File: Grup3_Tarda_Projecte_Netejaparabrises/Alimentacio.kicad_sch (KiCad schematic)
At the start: 12 parts, among them J1 Screw_Terminal_01x02, U1 LM1117-ADJ, U1 LM1117MP-5.0

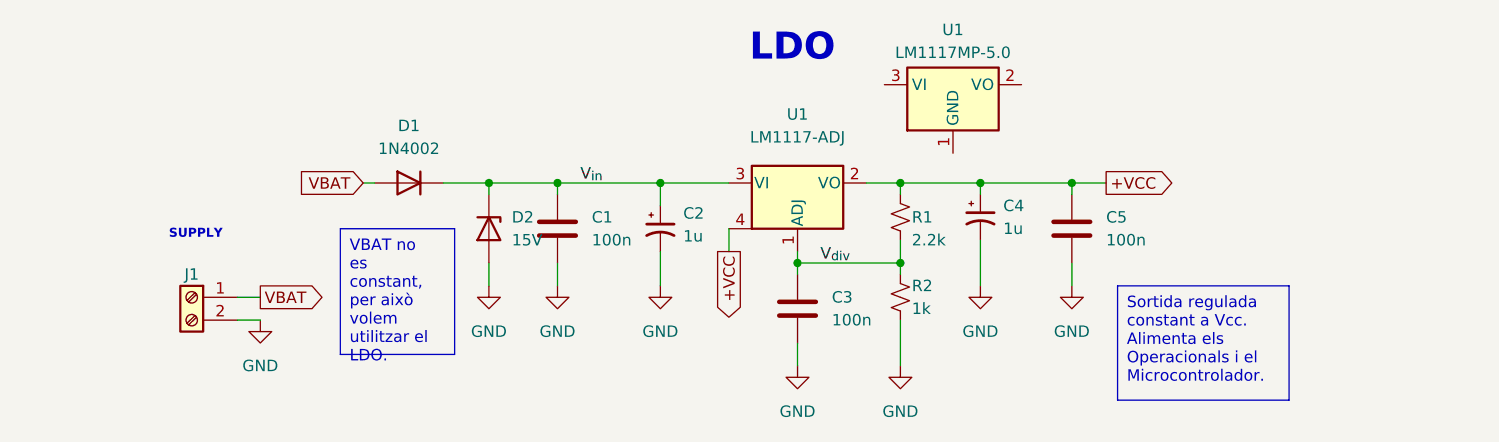
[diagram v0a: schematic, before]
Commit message: canvis esquematic
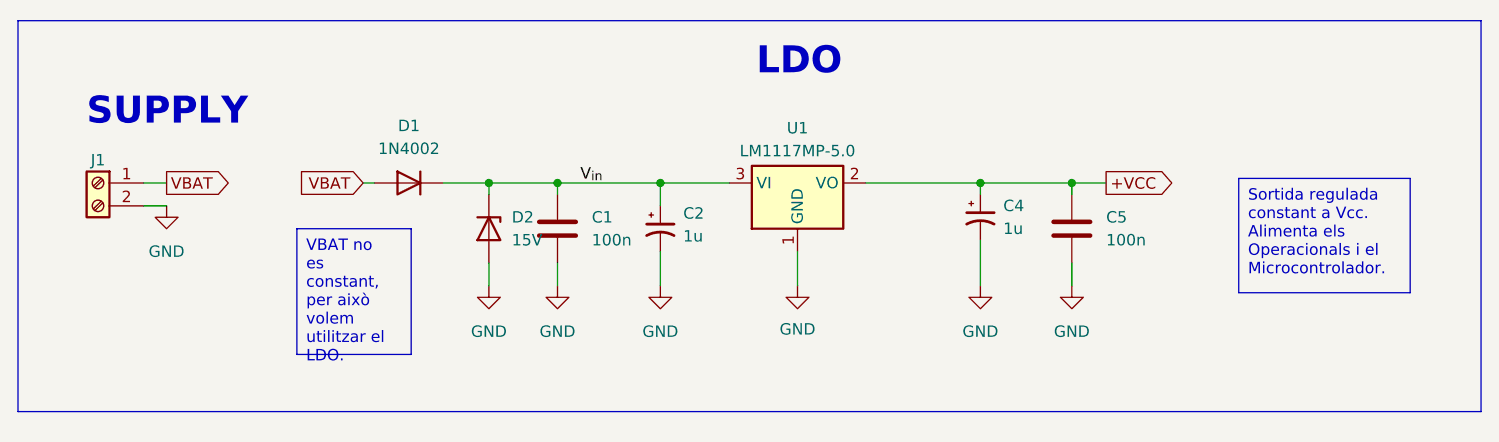
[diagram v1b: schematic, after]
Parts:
- removed C3: 100n, Capacitor_SMD:C_0805_2012Metric, symbol Device:C
- removed R1: 2.2k, Resistor_SMD:R_0805_2012Metric, symbol Device:R_Small_US
- removed R2: 1k, Resistor_SMD:R_0805_2012Metric, symbol Device:R_Small_US
- removed U1: LM1117-ADJ, Package_TO_SOT_THT:TO-220-3_Horizontal_TabDown, symbol Regulator_Linear:LM1117-ADJ
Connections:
- net +VCC: now also U1.2 (VO)
- net GND: now also U1.1 (GND)
- net V_{in}: now also U1.3 (VI)
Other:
- moved on the sheet: J1, U1
